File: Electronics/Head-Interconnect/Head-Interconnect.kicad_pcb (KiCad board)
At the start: 2 copper layers, 55 x 54.5 mm, 18 parts, among them J1 Conn_Coaxial, J2 Conn_02x03_Odd_Even

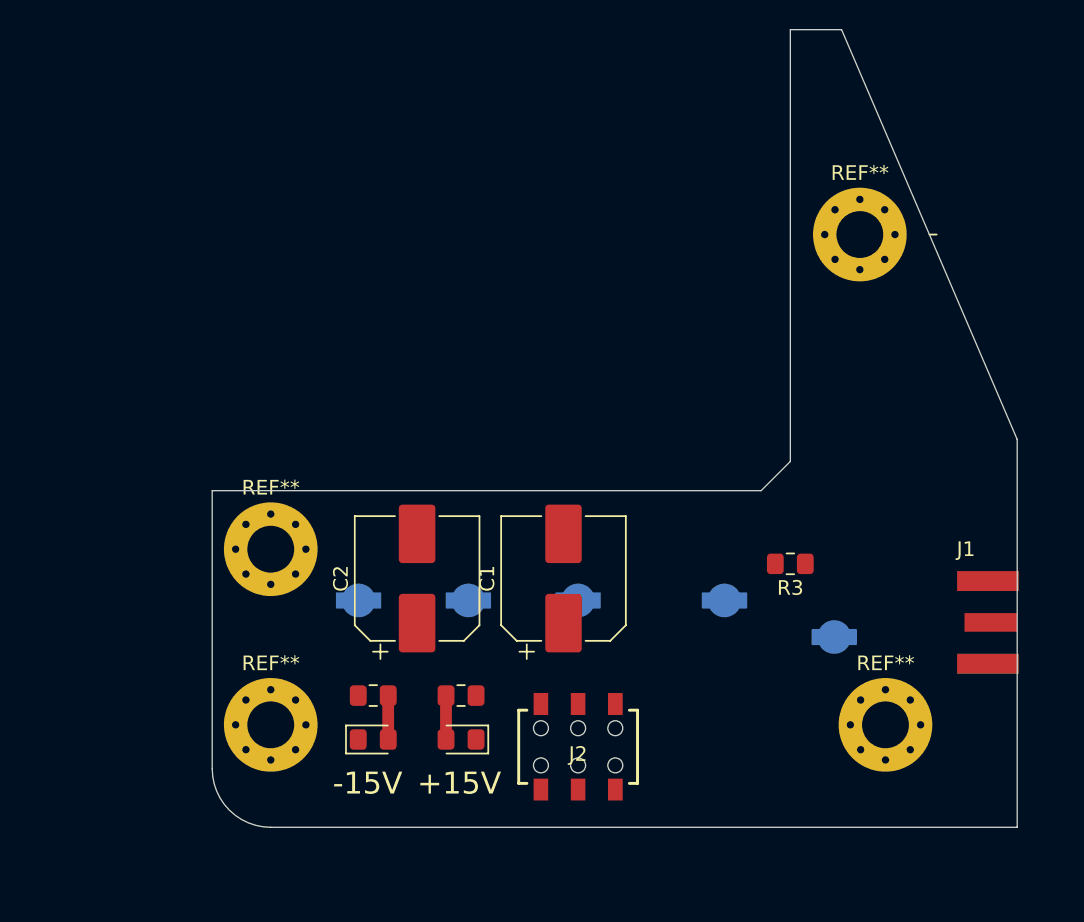
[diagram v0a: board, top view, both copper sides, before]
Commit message: Head interconnect finished
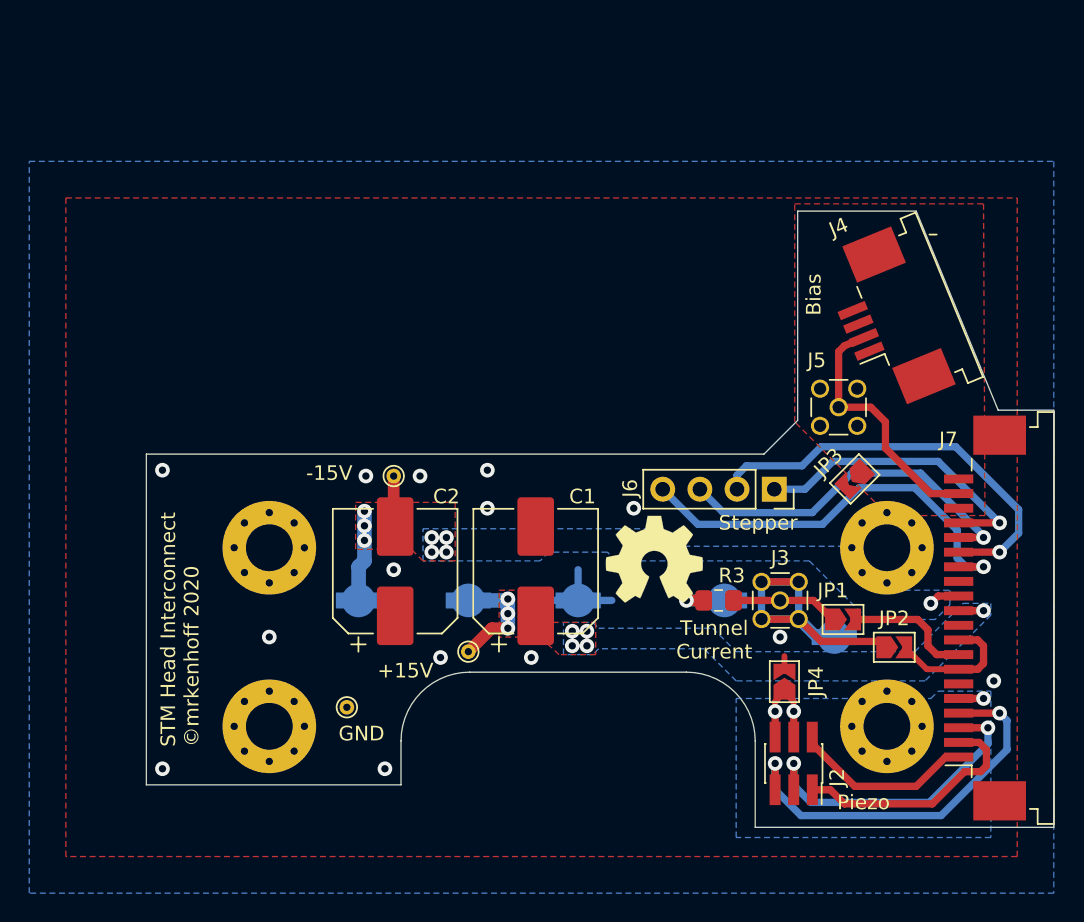
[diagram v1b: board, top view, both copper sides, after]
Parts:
- removed D1, D2: LED, LED_SMD:LED_0805_2012Metric_Pad1.15x1.40mm_HandSolder
- removed J1: Conn_Coaxial, Custom:SMA
- removed R1, R2: R, Resistor_SMD:R_0805_2012Metric_Pad1.15x1.40mm_HandSolder
- removed REF** (x4): MountingHole_3.2mm_M3_Pad_Via, MountingHole:MountingHole_3.2mm_M3_Pad_Via
- added H1: MountingHole_Pad, MountingHole:MountingHole_3.2mm_M3_Pad_Via, F.Cu at (126.4, 101.4)
- added H2: MountingHole_Pad, MountingHole:MountingHole_3.2mm_M3_Pad_Via, F.Cu at (126.4, 113.6)
- added H3: MountingHole_Pad, MountingHole:MountingHole_3.2mm_M3_Pad_Via, F.Cu at (168.6, 101.4)
- added H4: MountingHole_Pad, MountingHole:MountingHole_3.2mm_M3_Pad_Via, F.Cu at (168.6, 113.6)
- added J3: Conn_Coaxial, Connector_Coaxial:MMCX_Molex_73415-1471_Vertical, F.Cu at (161.3, 105.0)
- added J4: Conn_01x04_MountingPin, Connector_FFC-FPC:TE_84953-4_1x04-1MP_P1.0mm_Horizontal, F.Cu at (168.5, 85.9)
- added J5: Conn_Coaxial, Connector_Coaxial:MMCX_Molex_73415-1471_Vertical, F.Cu at (165.3, 91.8)
- added J6: Conn_01x04, Connector_PinSocket_2.54mm:PinSocket_1x04_P2.54mm_Vertical, F.Cu at (160.9, 97.4)
- added J7: Conn_01x20_MountingPin, Connector_FFC-FPC:TE_2-84953-0_1x20-1MP_P1.0mm_Horizontal, F.Cu at (175.3, 106.2)
- added JP1: Jumper, Jumper:SolderJumper-2_P1.3mm_Open_TrianglePad1.0x1.5mm, F.Cu at (165.6, 106.3)
- added JP2: Jumper, Jumper:SolderJumper-2_P1.3mm_Open_TrianglePad1.0x1.5mm, F.Cu at (169.1, 108.2)
- added JP3: Jumper, Jumper:SolderJumper-2_P1.3mm_Open_TrianglePad1.0x1.5mm, F.Cu at (166.4, 96.7)
- added JP4: Jumper, Jumper:SolderJumper-2_P1.3mm_Open_TrianglePad1.0x1.5mm, F.Cu at (161.6, 110.5)
- added LOGO1: Logo_Open_Hardware_Small, Symbol:OSHW-Symbol_6.7x6mm_SilkScreen, F.Cu at (152.7, 102.2)
- added TP6: TestPoint, TestPoint:TestPoint_THTPad_D1.0mm_Drill0.5mm, F.Cu at (140.0, 108.5)
- added TP7: TestPoint, TestPoint:TestPoint_THTPad_D1.0mm_Drill0.5mm, F.Cu at (131.7, 112.3)
- added TP8: TestPoint, TestPoint:TestPoint_THTPad_D1.0mm_Drill0.5mm, F.Cu at (134.9, 96.5)
- J2: footprint Custom:board-to-board -> Connector_PinSocket_1.27mm:PinSocket_2x03_P1.27mm_Vertical_SMD
- moved J2 14.8 mm to (162.2, 116.1), turned to 270 degrees
- moved R3 5.50 mm to (157.1, 105.0)
- moved C1 1.96 mm to (144.6, 103.0)
- moved C2 1.58 mm to (135.0, 103.0)
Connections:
- net +15V renamed /analog_+15V
- net -15V renamed /analog_-15V
- net GND renamed /analog_gnd
- J2 pad 1: Net-(J2-Pad1) -> /piezo_x-
- J2 pad 2: Net-(J2-Pad2) -> /piezo_x+
- J2 pad 3: Net-(J2-Pad3) -> /piezo_y+
- J2 pad 4: Net-(J2-Pad4) -> /piezo_gnd
- J2 pad 5: Net-(J2-Pad5) -> /piezo_y-
- J2 pad 6: Net-(J2-Pad6) -> /piezo_gnd
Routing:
- net /Stepper_A2: track 0.00 -> 29.0 mm, vias 0 -> 1
- net /Stepper_B2: track 0.00 -> 29.0 mm, vias 0 -> 1
- net /piezo_y-: track 0.00 -> 27.5 mm, vias 0 -> 2
- net /tunnel_gnd: track 0.00 -> 24.8 mm
- net /Stepper_B1: track 0.00 -> 24.7 mm, vias 0 -> 1
- net /piezo_y+: track 0.00 -> 21.8 mm, vias 0 -> 2
- net /Stepper_A1: track 0.00 -> 20.7 mm, vias 0 -> 1
- net /bias: track 0.00 -> 17.5 mm
- net /piezo_x-: track 0.00 -> 16.6 mm
- net /piezo_x+: track 0.00 -> 12.5 mm
- net /analog_-15V: track 0.00 -> 11.9 mm, vias 0 -> 8
- net /analog_+15V: track 0.00 -> 9.80 mm, vias 0 -> 8
- net /tunnel_gnd_ffc: track 0.00 -> 9.23 mm
- net /tunnel_signal_ffc: track 0.00 -> 8.81 mm
- net /piezo_gnd: track 0.00 -> 8.35 mm, vias 0 -> 3
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- added copper zone on B.Cu, net /analog_+15V
- added copper zone on F.Cu, net /analog_+15V
- added copper zone on B.Cu, net /analog_-15V
- added copper zone on F.Cu, net /analog_-15V
- added copper zone on B.Cu, net /analog_gnd
- added copper zone on F.Cu, net /analog_gnd
- added copper zone on F.Cu, net /bias_gnd
- added copper zone on B.Cu, net /piezo_gnd
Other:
- board size 55 x 54.5 mm -> 62 x 42.1 mm
- board text added: "Bias"
- board text added: "GND"
- board text added: "Gnd"
- board text added: "Piezo"
- board text added: "STM Head Interconnect"
- board text added: "Shield"
- board text added: "Sig"
- board text added: "Stepper"
- board text added: "Tunnel Current"
- board text added: "©mrkenhoff 2020"
